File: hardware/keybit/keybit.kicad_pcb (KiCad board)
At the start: 2 copper layers, 19 x 19 mm, 23 parts, among them SW1 SW_Push, U1 CH32V003FxUx, U2 YZ13515055F-02025-02, U3 YZ13515055F-02025-02, U4 YZ13515055F-02025-02, U5 YZ13515055F-02025-02, U6 YZ13515055F-02025-02, U7 YZ13515055F-02025-02, U8 YZ13515055F-02025-02, U9 YZ13515055F-02025-02

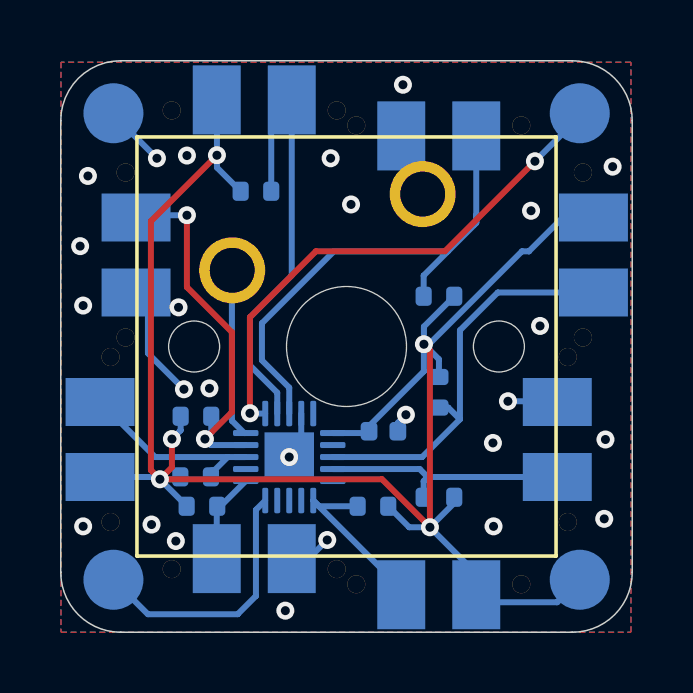
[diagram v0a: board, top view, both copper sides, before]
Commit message: fixes adn stuff
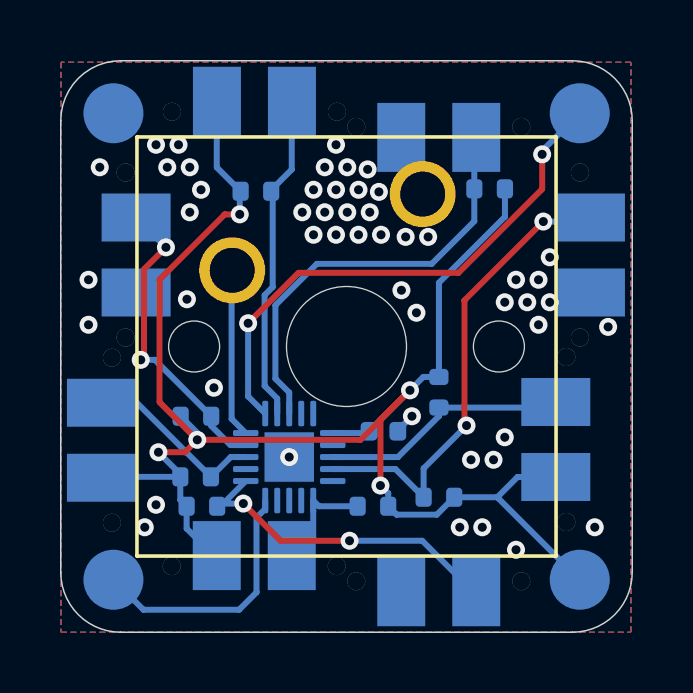
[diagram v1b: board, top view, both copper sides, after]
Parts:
- R1, R11, R2, R3, R4, R5, R6, R8: value 4.7K -> 10K
- moved R4 3.96 mm to (154.8, 70.9)
- moved U8 0.10 mm to (146.9, 83.1)
- moved U9 0.10 mm to (153.1, 84.3)
- moved U6 0.10 mm to (158.2, 73.1)
- moved U4 0.05 mm to (141.8, 79.3)
- moved U3 0.05 mm to (153.1, 69.2)
- moved U7 0.05 mm to (157.0, 79.3)
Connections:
- U6 pad 1: +3.3V -> /SCL2
- U6 pad 2: /SDA2 -> GND
- U7 pad 1: /SCL2 -> +3.3V
- U7 pad 2: GND -> /SDA2
- U8 pad 1: /SCL1 -> +3.3V
- U8 pad 2: GND -> /SDA1
- U9 pad 1: +3.3V -> /SCL1
- U9 pad 2: /SDA1 -> GND
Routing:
- net GND: track 12.2 -> 0.69 mm, vias 26 -> 50
- net /SCL1: track 2.99 -> 11.2 mm, vias 0 -> 2
- net /SCL2: track 8.33 -> 16.0 mm, vias 0 -> 2
- net +3.3V: track 62.8 -> 56.9 mm
- net /SDA2: track 13.6 -> 8.41 mm
- net /SDA4: track 14.7 -> 11.0 mm
- net /SCL4: track 16.9 -> 14.5 mm
- net /SDA1: track 5.91 -> 3.79 mm
- net /SCL3: track 12.5 -> 10.4 mm
